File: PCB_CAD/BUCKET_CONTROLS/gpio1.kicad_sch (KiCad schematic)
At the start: 13 parts, among them U12 MCP23017_I2C2_0x20, U13 MCP23017_I2C2_0x21, U14 MCP23017_I2C2_0x22

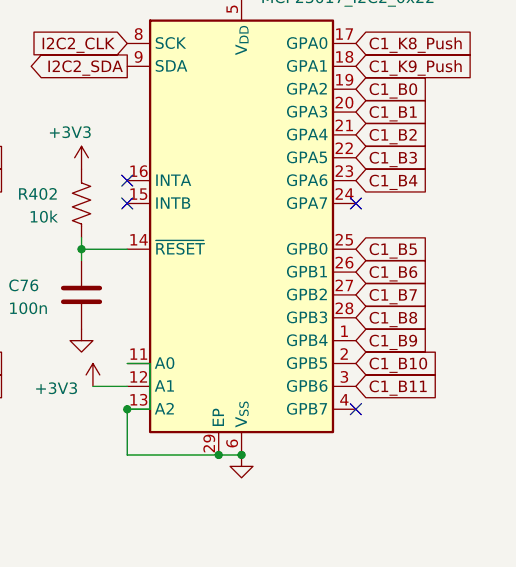
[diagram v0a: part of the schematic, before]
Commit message: pcb routing all day
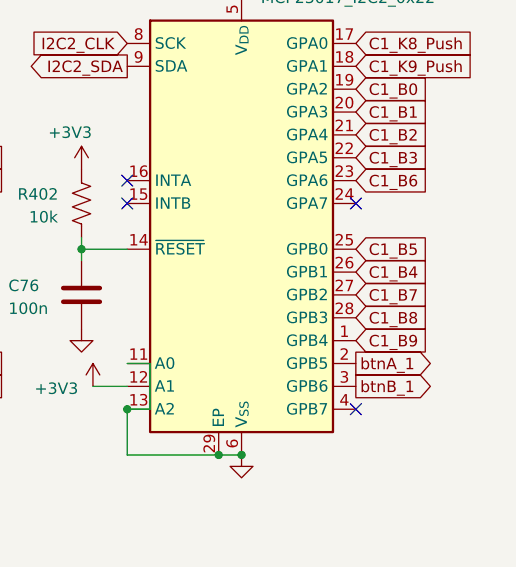
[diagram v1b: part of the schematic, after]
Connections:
- net C1_B4: now also U14.26 (GPB1); no longer U14.23 (GPA6)
- net C1_B6: now also U14.23 (GPA6); no longer U14.26 (GPB1)
- net C1_B10 renamed btnA_1
- net C1_B11 renamed btnB_1
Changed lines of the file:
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@@
 	(global_label "C1_B4"
 		(shape input)
-		(at 205.74 72.39 0)
-		(fields_autoplaced yes)
-		(effects
-			(font
-				(size 1.27 1.27)
-			)
-			(justify left)
-		)
-		(property "Intersheetrefs" "${INTERSHEET_REFS}"
-			(at 214.6518 72.39 0)
+		(at 205.74 82.55 0)
+		(fields_autoplaced yes)
+		(effects
+			(font
+				(size 1.27 1.27)
+			)
+			(justify left)
+		)
+		(property "Intersheetrefs" "${INTERSHEET_REFS}"
+			(at 214.6518 82.55 0)
 			(hide yes)
 			(show_name no)
@@
 		)
 	)
-	(global_label "C1_B11"
-		(shape input)
-		(at 205.74 95.25 0)
-		(fields_autoplaced yes)
-		(effects
-			(font
-				(size 1.27 1.27)
-			)
-			(justify left)
-		)
-		(property "Intersheetrefs" "${INTERSHEET_REFS}"
-			(at 215.8613 95.25 0)
+	(global_label "btnA_1"
+		(shape output)
+		(at 205.74 92.71 0)
+		(fields_autoplaced yes)
+		(effects
+			(font
+				(size 1.27 1.27)
+				(color 255 255 255 1)
+			)
+			(justify left)
+		)
+		(property "Intersheetrefs" "${INTERSHEET_REFS}"
+			(at 215.0146 92.71 0)
 			(hide yes)
 			(show_name no)
@@
 		)
 	)
-	(global_label "C1_B10"
-		(shape input)
-		(at 205.74 92.71 0)
-		(fields_autoplaced yes)
-		(effects
-			(font
-				(size 1.27 1.27)
-			)
-			(justify left)
-		)
-		(property "Intersheetrefs" "${INTERSHEET_REFS}"
-			(at 215.8613 92.71 0)
+	(global_label "btnB_1"
+		(shape output)
+		(at 205.74 95.25 0)
+		(fields_autoplaced yes)
+		(effects
+			(font
+				(size 1.27 1.27)
+				(color 255 255 255 1)
+			)
+			(justify left)
+		)
+		(property "Intersheetrefs" "${INTERSHEET_REFS}"
+			(at 215.196 95.25 0)
 			(hide yes)
 			(show_name no)
@@
 	(global_label "C1_B6"
 		(shape input)
-		(at 205.74 82.55 0)
-		(fields_autoplaced yes)
-		(effects
-			(font
-				(size 1.27 1.27)
-			)
-			(justify left)
-		)
-		(property "Intersheetrefs" "${INTERSHEET_REFS}"
-			(at 214.6518 82.55 0)
-			(hide yes)
-			(show_name no)
+		(at 205.74 72.39 0)
+		(fields_autoplaced yes)
+		(effects
+			(font
+				(size 1.27 1.27)
+			)
+			(justify left)
+		)
+		(property "Intersheetrefs" "${INTERSHEET_REFS}"
+			(at 214.6518 72.39 0)
+			(hide yes)
+			(show_name no)
